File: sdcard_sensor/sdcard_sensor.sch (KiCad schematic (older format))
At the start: 1 part, among them X1 microSD_Card

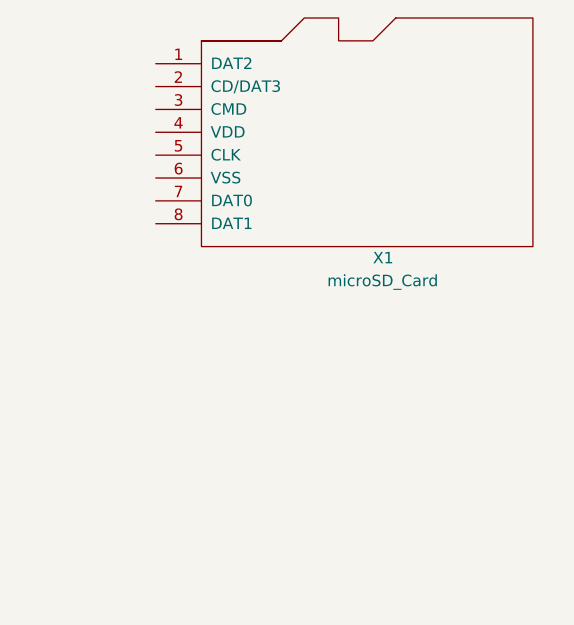
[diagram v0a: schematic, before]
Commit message: Template done
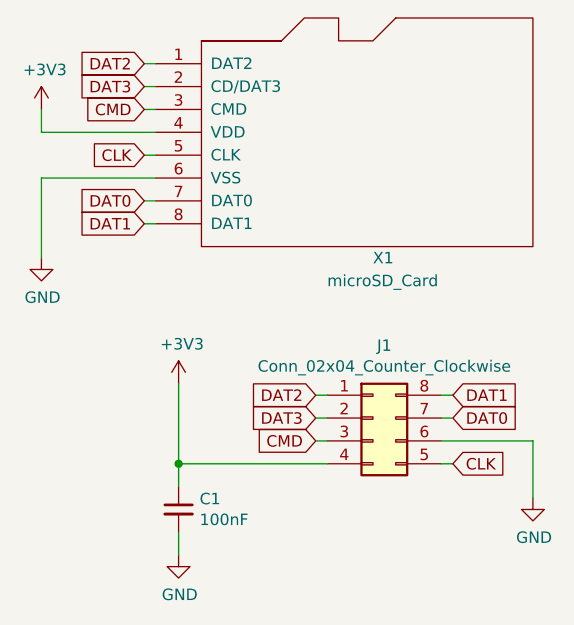
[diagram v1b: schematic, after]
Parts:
- added C1: 100nF, Capacitor_SMD:C_0402_1005Metric, symbol Device:C_Small
- added J1: Conn_02x04_Counter_Clockwise, Connector_PinSocket_2.00mm:PinSocket_2x04_P2.00mm_Vertical, symbol Connector_Generic:Conn_02x04_Counter_Clockwise
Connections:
- net DAT2: now reaches X1.1 (DAT2)
- net DAT2: now also J1.1 (Pin_1)
- net DAT3: now reaches X1.2 (CD/DAT3)
- net DAT3: now also J1.2 (Pin_2)
- net CMD: now reaches X1.3 (CMD)
- net CMD: now also J1.3 (Pin_3)
- net +3V3: now reaches X1.4 (VDD)
- net +3V3: now also C1.1, J1.4 (Pin_4)
- net CLK: now reaches X1.5 (CLK)
- net CLK: now also J1.5 (Pin_5)
- net GND: now reaches X1.6 (VSS)
- net GND: now also C1.2, J1.6 (Pin_6)
- net DAT0: now reaches X1.7 (DAT0)
- net DAT0: now also J1.7 (Pin_7)
- net DAT1: now reaches X1.8 (DAT1)
- net DAT1: now also J1.8 (Pin_8)
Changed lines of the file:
@@
 encoding utf-8
 Sheet 1 1
-Title ""
-Date ""
-Rev ""
-Comp ""
+Title "MicroSD Sensor Module"
+Date "2021-02-21"
+Rev "0.1"
+Comp "Pedro Minatel"
 Comment1 ""
 Comment2 ""
@@
 	1    0    0    -1
 $EndComp
+$Comp
+L Connector_Generic:Conn_02x04_Counter_Clockwise J1
+U 1 1 6032826B
+P 9600 2800
+F 0 "J1" H 9650 3117 50  0000 C CNN
+F 1 "Conn_02x04_Counter_Clockwise" H 9650 3026 50  0000 C CNN
+F 2 "Connector_PinSocket_2.00mm:PinSocket_2x04_P2.00mm_Vertical" H 9600 2800 50  0001 C CNN
+F 3 "~" H 9600 2800 50  0001 C CNN
+	1    9600 2800
+	1    0    0    -1
+$EndComp
+Text GLabel 8600 1250 0    50   Input ~ 0
+DAT2
+Text GLabel 8600 1350 0    50   Input ~ 0
+DAT3
+Text GLabel 8600 1450 0    50   Input ~ 0
+CMD
+Text GLabel 8600 1650 0    50   Input ~ 0
+CLK
+Text GLabel 8600 1850 0    50   Input ~ 0
+DAT0
+Text GLabel 8600 1950 0    50   Input ~ 0
+DAT1
+Wire Wire Line
+	8600 1950 8650 1950
+Wire Wire Line
+	8600 1850 8650 1850
+Wire Wire Line
+	8600 1650 8650 1650
+Wire Wire Line
+	8600 1450 8650 1450
+Wire Wire Line
+	8600 1350 8650 1350
+Wire Wire Line
+	8600 1250 8650 1250
+Text GLabel 9350 2700 0    50   Input ~ 0
+DAT2
+Text GLabel 9350 2800 0    50   Input ~ 0
+DAT3
+Text GLabel 9350 2900 0    50   Input ~ 0
+CMD
+Text GLabel 9950 3000 2    50   Input ~ 0
+CLK
+Text GLabel 9950 2800 2    50   Input ~ 0
+DAT0
+Text GLabel 9950 2700 2    50   Input ~ 0
+DAT1
+Wire Wire Line
+	9900 2700 9950 2700
+Wire Wire Line
+	9900 2800 9950 2800
+Wire Wire Line
+	9900 3000 9950 3000
+Wire Wire Line
+	9350 2900 9400 2900
+Wire Wire Line
+	9350 2800 9400 2800
+Wire Wire Line
+	9350 2700 9400 2700
+$Comp
+L power:GND #PWR05
+U 1 1 60334059
+P 10300 3150
+F 0 "#PWR05" H 10300 2900 50  0001 C CNN
+F 1 "GND" H 10305 2977 50  0000 C CNN
+F 2 "" H 10300 3150 50  0001 C CNN
+F 3 "" H 10300 3150 50  0001 C CNN
+	1    10300 3150
+	1    0    0    -1
+$EndComp
+$Comp
+L power:+3V3 #PWR03
+U 1 1 603344EE
+P 8750 2650
+F 0 "#PWR03" H 8750 2500 50  0001 C CNN
+F 1 "+3V3" H 8765 2823 50  0000 C CNN
+F 2 "" H 8750 2650 50  0001 C CNN
+F 3 "" H 8750 2650 50  0001 C CNN
+	1    8750 2650
+	1    0    0    -1
+$EndComp
+$Comp
+L power:+3V3 #PWR01
+U 1 1 6033B7FD
+P 8150 1450
+F 0 "#PWR01" H 8150 1300 50  0001 C CNN
+F 1 "+3V3" H 8165 1623 50  0000 C CNN
+F 2 "" H 8150 1450 50  0001 C CNN
+F 3 "" H 8150 1450 50  0001 C CNN
+	1    8150 1450
+	1    0    0    -1
+$EndComp
+$Comp
+L power:GND #PWR02
+U 1 1 6033C0A3
+P 8150 2100
+F 0 "#PWR02" H 8150 1850 50  0001 C CNN
+F 1 "GND" H 8155 1927 50  0000 C CNN
+F 2 "" H 8150 2100 50  0001 C CNN
+F 3 "" H 8150 2100 50  0001 C CNN
+	1    8150 2100
+	1    0    0    -1
+$EndComp
+Wire Wire Line
+	8150 1550 8150 1450
+Wire Wire Line
+	8150 1550 8650 1550
+Wire Wire Line
+	8150 1750 8150 2100
+Wire Wire Line
+	8150 1750 8650 1750
+Wire Wire Line
+	8750 2650 8750 3000
+Wire Wire Line
+	8750 3000 9400 3000
+Wire Wire Line
+	10300 2900 10300 3150
+Wire Wire Line
+	9900 2900 10300 2900
+$Comp
+L Device:C_Small C1
+U 1 1 60340E34
+P 8750 3200
+F 0 "C1" H 8842 3246 50  0000 L CNN
+F 1 "100nF" H 8842 3155 50  0000 L CNN
+F 2 "Capacitor_SMD:C_0402_1005Metric" H 8750 3200 50  0001 C CNN
+F 3 "~" H 8750 3200 50  0001 C CNN
+	1    8750 3200
+	1    0    0    -1
+$EndComp
+$Comp
+L power:GND #PWR04
+U 1 1 60341321
+P 8750 3400
+F 0 "#PWR04" H 8750 3150 50  0001 C CNN
+F 1 "GND" H 8755 3227 50  0000 C CNN
+F 2 "" H 8750 3400 50  0001 C CNN
+F 3 "" H 8750 3400 50  0001 C CNN
+	1    8750 3400
+	1    0    0    -1
+$EndComp
+Wire Wire Line
+	8750 3100 8750 3000
+Connection ~ 8750 3000
+Wire Wire Line
+	8750 3400 8750 3300
 $EndSCHEMATC
